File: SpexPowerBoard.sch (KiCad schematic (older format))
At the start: 12 parts

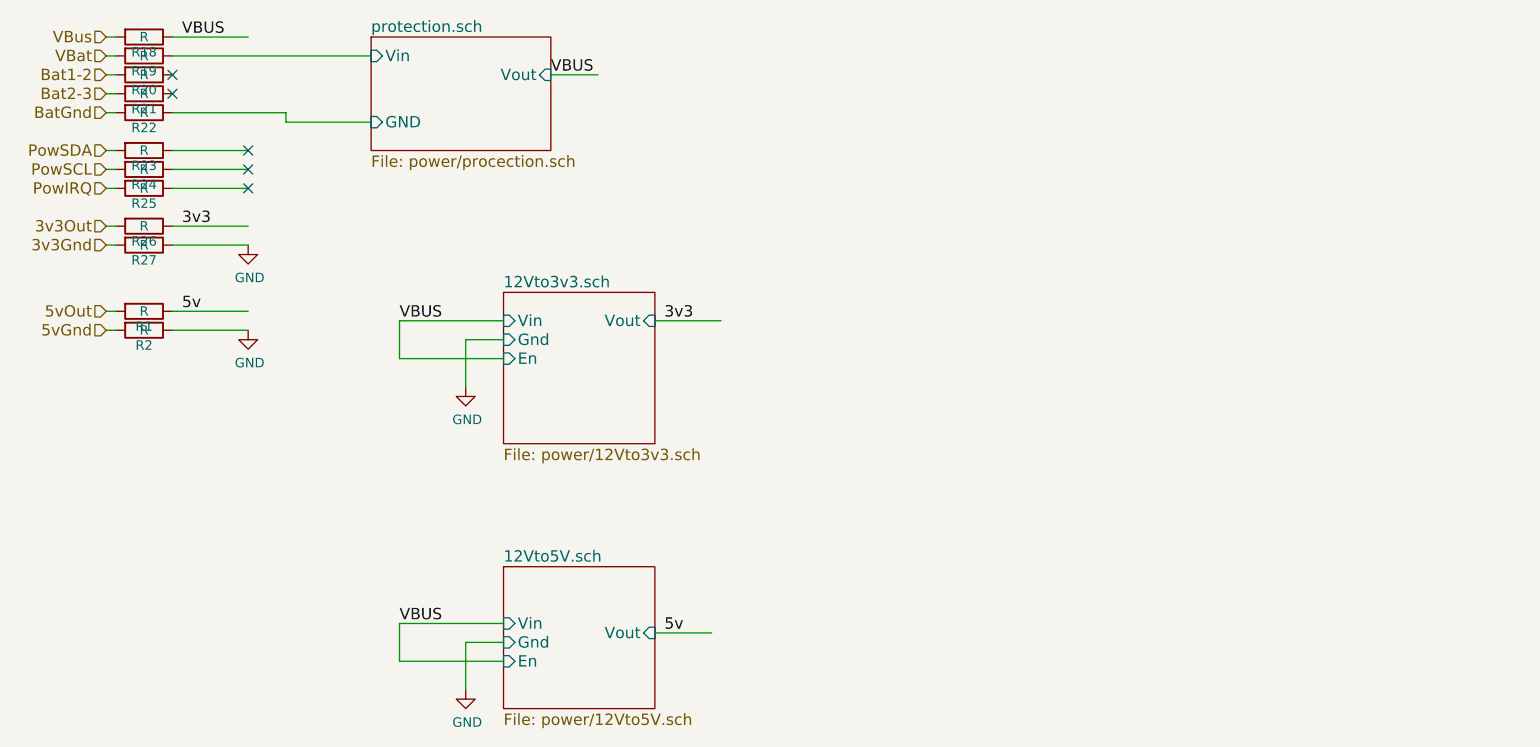
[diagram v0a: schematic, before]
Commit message: working on PCB layout
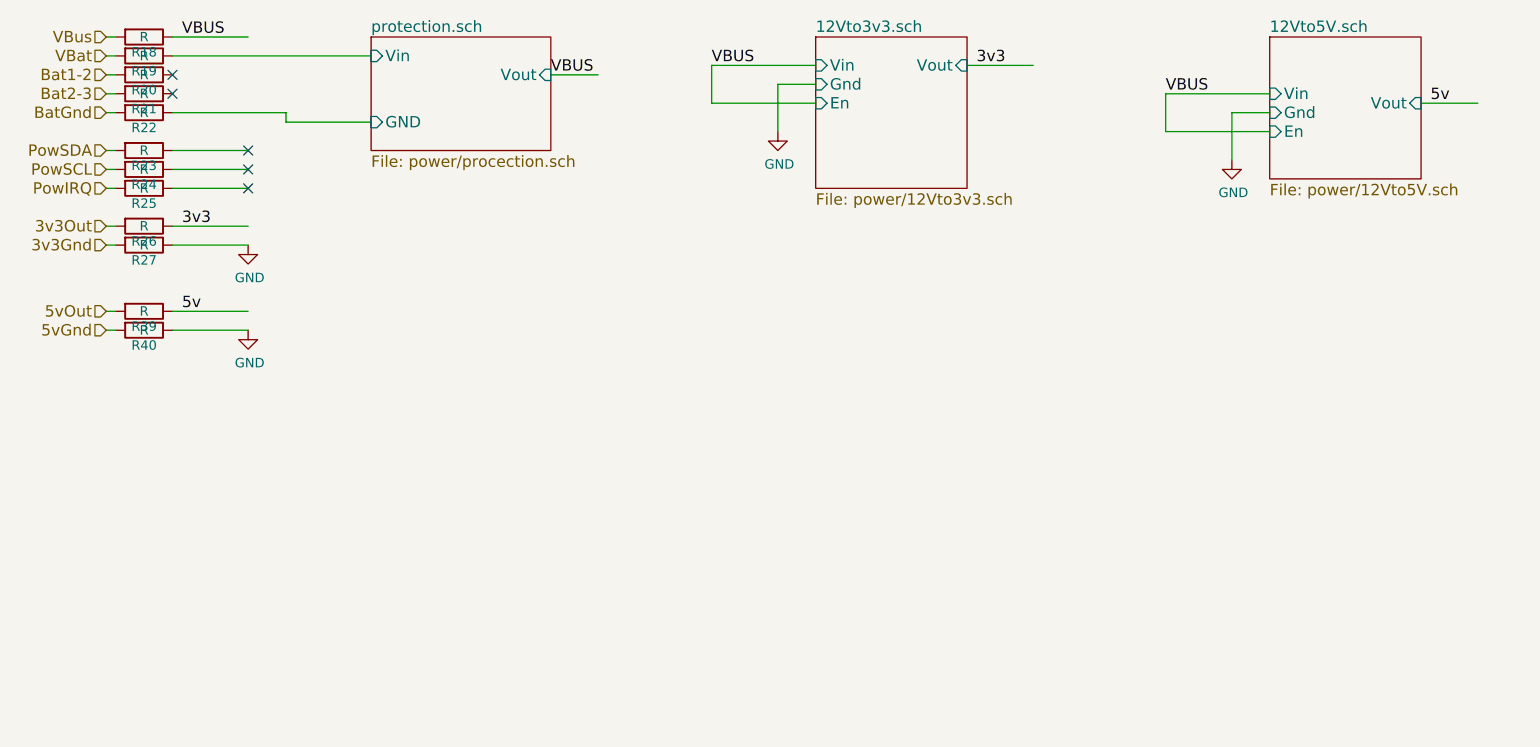
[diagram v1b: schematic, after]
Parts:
- renumbered R1 to R39, R2 to R40
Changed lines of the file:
@@
 LIBS:contrib
 LIBS:valves
+LIBS:parts
+LIBS:PRESSURE-BMP180_LGA7_
+LIBS:74xgxx
+LIBS:ac-dc
+LIBS:actel
+LIBS:Altera
+LIBS:analog_devices
+LIBS:brooktre
+LIBS:cmos_ieee
+LIBS:dc-dc
+LIBS:diode
+LIBS:elec-unifil
+LIBS:ESD_Protection
+LIBS:ftdi
+LIBS:gennum
+LIBS:graphic
+LIBS:hc11
+LIBS:ir
+LIBS:Lattice
+LIBS:logo
+LIBS:maxim
+LIBS:microchip_dspic33dsc
+LIBS:microchip_pic10mcu
+LIBS:microchip_pic12mcu
+LIBS:microchip_pic16mcu
+LIBS:microchip_pic18mcu
+LIBS:microchip_pic32mcu
+LIBS:motor_drivers
+LIBS:msp430
+LIBS:nordicsemi
+LIBS:nxp_armmcu
+LIBS:onsemi
+LIBS:Oscillators
+LIBS:Power_Management
+LIBS:powerint
+LIBS:pspice
+LIBS:references
+LIBS:relays
+LIBS:rfcom
+LIBS:sensors
+LIBS:silabs
+LIBS:stm8
+LIBS:stm32
+LIBS:supertex
+LIBS:switches
+LIBS:transf
+LIBS:ttl_ieee
+LIBS:video
+LIBS:Xicor
+LIBS:Zilog
 LIBS:KL03-QFN24
 LIBS:lt3652
@@
 LIBS:si3407dv
 LIBS:tps563200
-LIBS:diode
-LIBS:SpexPowerBoard-cache
+LIBS:Spex-Mainboard-Hardware-cache
 EELAYER 25 0
 EELAYER END
 $Descr A4 11693 8268
 encoding utf-8
-Sheet 1 4
+Sheet 3 7
 Title ""
 Date ""
@@
 $EndComp
 $Sheet
-S 4050 2150 800  800
+S 5700 800  800  800
 U 56FE3A4E
 F0 "12Vto3v3.sch" 60
 F1 "power/12Vto3v3.sch" 60
-F2 "Vin" I L 4050 2300 60
-F3 "Gnd" I L 4050 2400 60
-F4 "En" I L 4050 2500 60
-F5 "Vout" I R 4850 2300 60
+F2 "Vin" I L 5700 950 60
+F3 "Gnd" I L 5700 1050 60
+F4 "En" I L 5700 1150 60
+F5 "Vout" I R 6500 950 60
 $EndSheet
 $Sheet
@@
 Text Label 4300 1000 0    60   ~ 0
 VBUS
-Text Label 3500 2300 0    60   ~ 0
+Text Label 5150 950  0    60   ~ 0
 VBUS
 $Comp
-L GND #PWR3
+L GND #PWR056
 U 1 1 56FE58A8
-P 3850 2650
-F 0 "#PWR3" H 3850 2400 50  0001 C CNN
-F 1 "GND" H 3858 2477 50  0000 C CNN
-F 2 "" H 3850 2650 50  0000 C CNN
-F 3 "" H 3850 2650 50  0000 C CNN
-	1    3850 2650
+P 5500 1300
+F 0 "#PWR056" H 5500 1050 50  0001 C CNN
+F 1 "GND" H 5508 1127 50  0000 C CNN
+F 2 "" H 5500 1300 50  0000 C CNN
+F 3 "" H 5500 1300 50  0000 C CNN
+	1    5500 1300
 	1    0    0    -1
 $EndComp
@@
 	4300 1000 4550 1000
 Wire Wire Line
-	4050 2300 3500 2300
-Wire Wire Line
-	4050 2500 3500 2500
-Wire Wire Line
-	3500 2500 3500 2300
-Wire Wire Line
-	3850 2400 4050 2400
-Wire Wire Line
-	3850 2400 3850 2650
-Wire Wire Line
-	4850 2300 5200 2300
-Text Label 4900 2300 0    60   ~ 0
+	5700 950  5150 950
+Wire Wire Line
+	5700 1150 5150 1150
+Wire Wire Line
+	5150 1150 5150 950
+Wire Wire Line
+	5500 1050 5700 1050
+Wire Wire Line
+	5500 1050 5500 1300
+Wire Wire Line
+	6500 950  6850 950
+Text Label 6550 950  0    60   ~ 0
 3v3
-Text Label 3500 3900 0    60   ~ 0
+Text Label 7550 1100 0    60   ~ 0
 VBUS
 $Comp
-L GND #PWR4
+L GND #PWR057
 U 1 1 56FE6215
-P 3850 4250
-F 0 "#PWR4" H 3850 4000 50  0001 C CNN
-F 1 "GND" H 3858 4077 50  0000 C CNN
-F 2 "" H 3850 4250 50  0000 C CNN
-F 3 "" H 3850 4250 50  0000 C CNN
-	1    3850 4250
+P 7900 1450
+F 0 "#PWR057" H 7900 1200 50  0001 C CNN
+F 1 "GND" H 7908 1277 50  0000 C CNN
+F 2 "" H 7900 1450 50  0000 C CNN
+F 3 "" H 7900 1450 50  0000 C CNN
+	1    7900 1450
 	1    0    0    -1
 $EndComp
 Wire Wire Line
-	4050 3900 3500 3900
-Wire Wire Line
-	4050 4100 3500 4100
-Wire Wire Line
-	3500 4100 3500 3900
-Wire Wire Line
-	3850 4000 4050 4000
-Wire Wire Line
-	3850 4000 3850 4250
+	8100 1100 7550 1100
+Wire Wire Line
+	8100 1300 7550 1300
+Wire Wire Line
+	7550 1300 7550 1100
+Wire Wire Line
+	7900 1200 8100 1200
+Wire Wire Line
+	7900 1200 7900 1450
 $Sheet
-S 4050 3600 800  750
+S 8100 800  800  750
 U 56FE62EA
 F0 "12Vto5V.sch" 60
 F1 "power/12Vto5V.sch" 60
-F2 "Vin" I L 4050 3900 60
-F3 "Gnd" I L 4050 4000 60
-F4 "En" I L 4050 4100 60
-F5 "Vout" I R 4850 3950 60
+F2 "Vin" I L 8100 1100 60
+F3 "Gnd" I L 8100 1200 60
+F4 "En" I L 8100 1300 60
+F5 "Vout" I R 8900 1150 60
 $EndSheet
 Wire Wire Line
-	4850 3950 5150 3950
-Text Label 4900 3950 0    60   ~ 0
+	8900 1150 9200 1150
+Text Label 8950 1150 0    60   ~ 0
 5v
 Wire Wire Line
@@
 3v3
 $Comp
-L GND #PWR1
+L GND #PWR058
 U 1 1 56FE74FE
 P 2700 1900
-F 0 "#PWR1" H 2700 1650 50  0001 C CNN
+F 0 "#PWR058" H 2700 1650 50  0001 C CNN
 F 1 "GND" H 2708 1727 50  0000 C CNN
 F 2 "" H 2700 1900 50  0000 C CNN
@@
 5vGnd
 $Comp
-L R R1
+L R R39
 U 1 1 56FE7B52
 P 2150 2250
-F 0 "R1" V 2230 2250 50  0000 C CNN
+F 0 "R39" V 2230 2250 50  0000 C CNN
 F 1 "R" V 2150 2250 50  0000 C CNN
 F 2 "Resistors_SMD:R_0603" V 2080 2250 50  0001 C CNN
@@
 $EndComp
 $Comp
-L R R2
+L R R40
 U 1 1 56FE7B58
 P 2150 2350
-F 0 "R2" V 2230 2350 50  0000 C CNN
+F 0 "R40" V 2230 2350 50  0000 C CNN
 F 1 "R" V 2150 2350 50  0000 C CNN
 F 2 "Resistors_SMD:R_0603" V 2080 2350 50  0001 C CNN
@@
 5v
 $Comp
-L GND #PWR2
+L GND #PWR059
 U 1 1 56FE7B63
 P 2700 2350
-F 0 "#PWR2" H 2700 2100 50  0001 C CNN
+F 0 "#PWR059" H 2700 2100 50  0001 C CNN
 F 1 "GND" H 2708 2177 50  0000 C CNN
 F 2 "" H 2700 2350 50  0000 C CNN
